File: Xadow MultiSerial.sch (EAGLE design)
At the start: 19 parts, among them J1 12p 0.5mm bottom contact, J2 12p 0.5mm bottom contact, J3 12p 0.5mm bottom contact, J4 12p 0.5mm bottom contact, U1 SC16IS752, X1 CTS_32X25_SMD

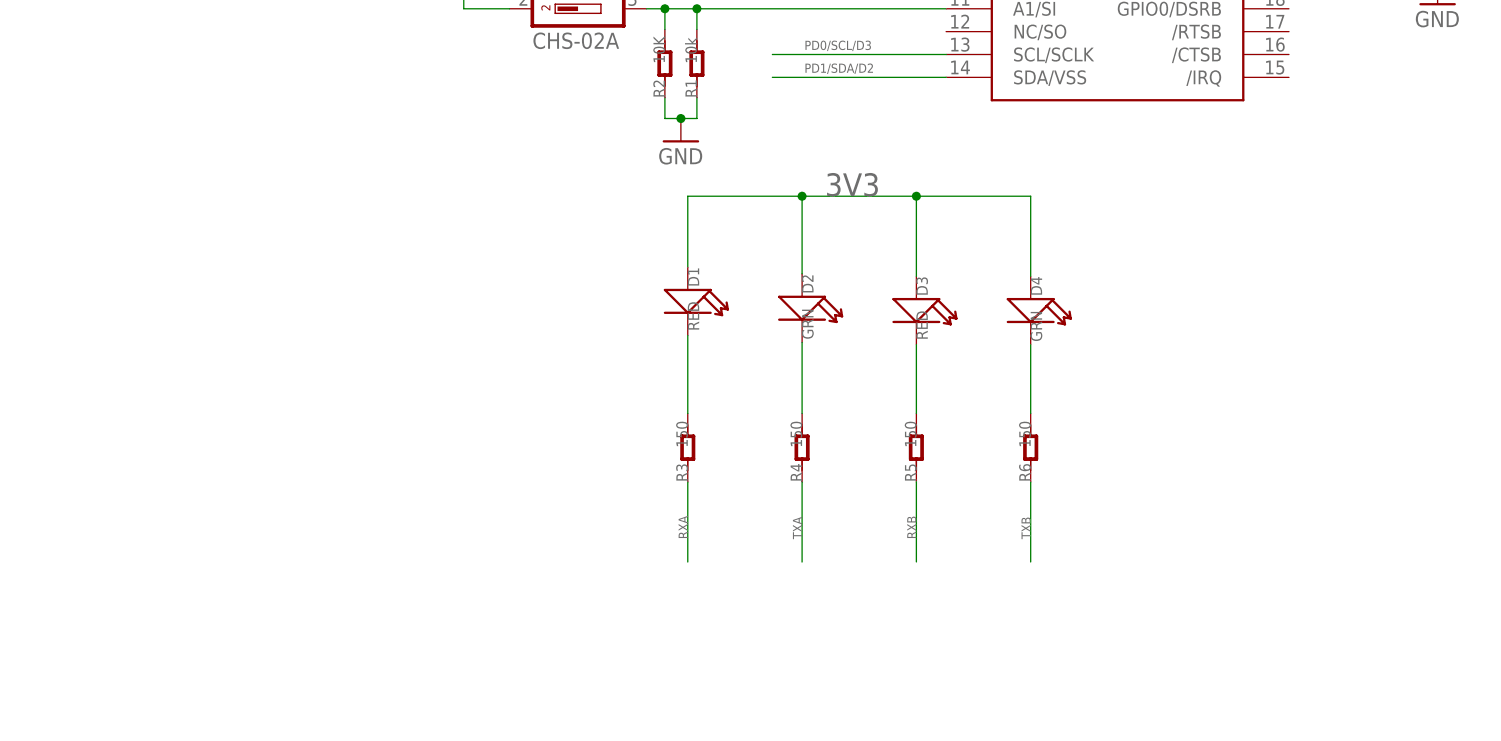
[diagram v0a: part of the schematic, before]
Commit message: Added level shifter MOSFETs
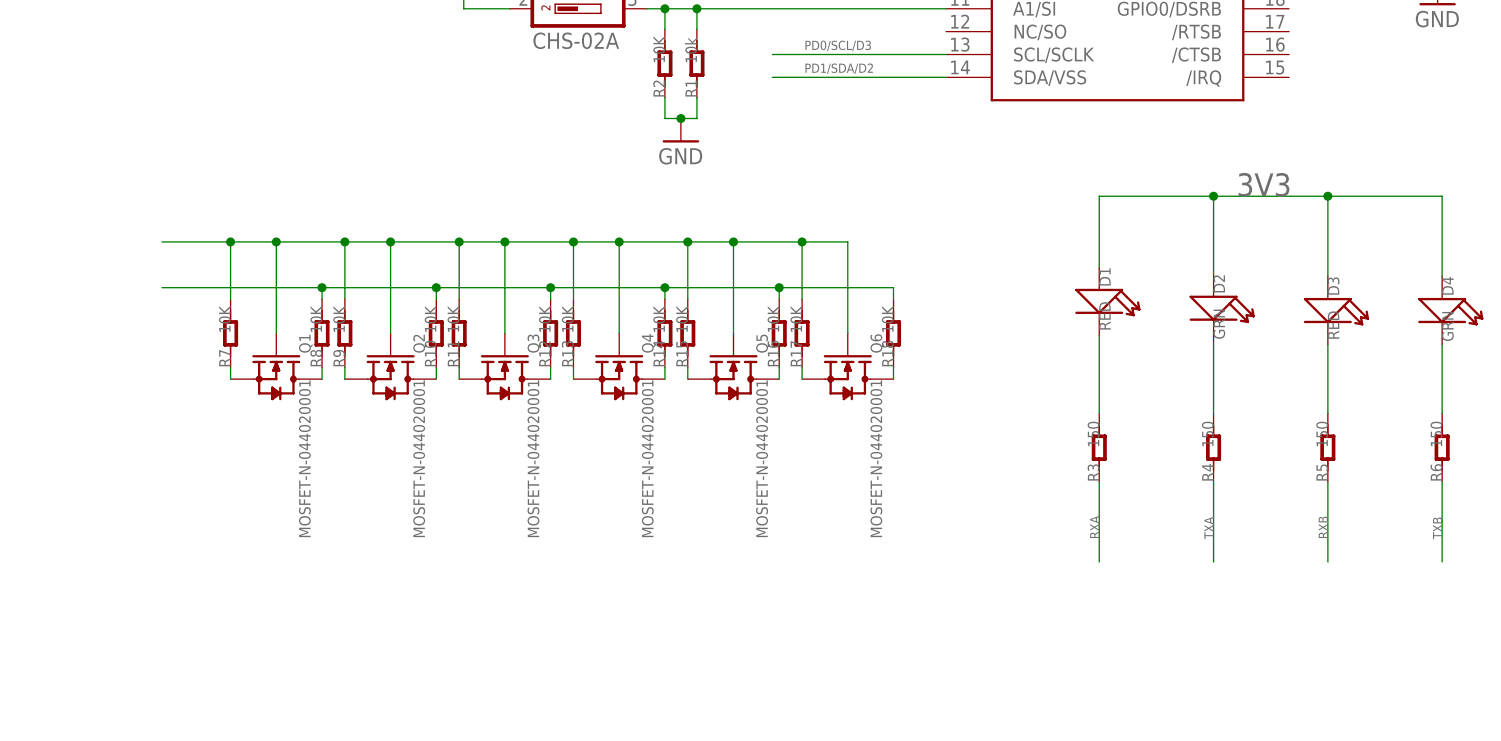
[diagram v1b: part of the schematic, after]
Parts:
- added Q1, Q2, Q3, Q4, Q5, Q6: MOSFET-N-044020001, OPL:MOSFET-N-044020001
- added R10, R11, R12, R13, R14, R15, R16, R17, R18, R7, R8, R9: 10K, OPL:R-0603
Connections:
- new net N$11: Q1.S, R7.1
- new net N$12: Q2.S, R9.1
- new net N$13: Q3.S, R11.1
- new net N$14: Q4.S, R13.1
- new net N$15: Q5.S, R15.1
- new net N$16: Q6.S, R17.1
- new net N$17: R10.2, R12.2, R14.2, R16.2, R18.2, R8.2
- new net N$18: Q1.D, R8.1
- new net N$19: Q2.D, R10.1
- new net N$20: Q3.D, R12.1
- new net N$21: Q4.D, R14.1
- new net N$22: Q5.D, R16.1
- new net N$23: Q6.D, R18.1
- new net N$4: Q1.G, Q2.G, Q3.G, Q4.G, Q5.G, Q6.G, R11.2, R13.2, R15.2, R17.2, R7.2, R9.2
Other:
- moved on the sheet: D1, D2, D3, D4, R3, R4, R5, R6
